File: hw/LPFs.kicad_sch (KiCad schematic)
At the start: 26 parts, among them K201 G6K-2, K202 G6K-2, K203 G6K-2, Q201 2N7002H, Q202 2N7002H, Q203 2N7002H

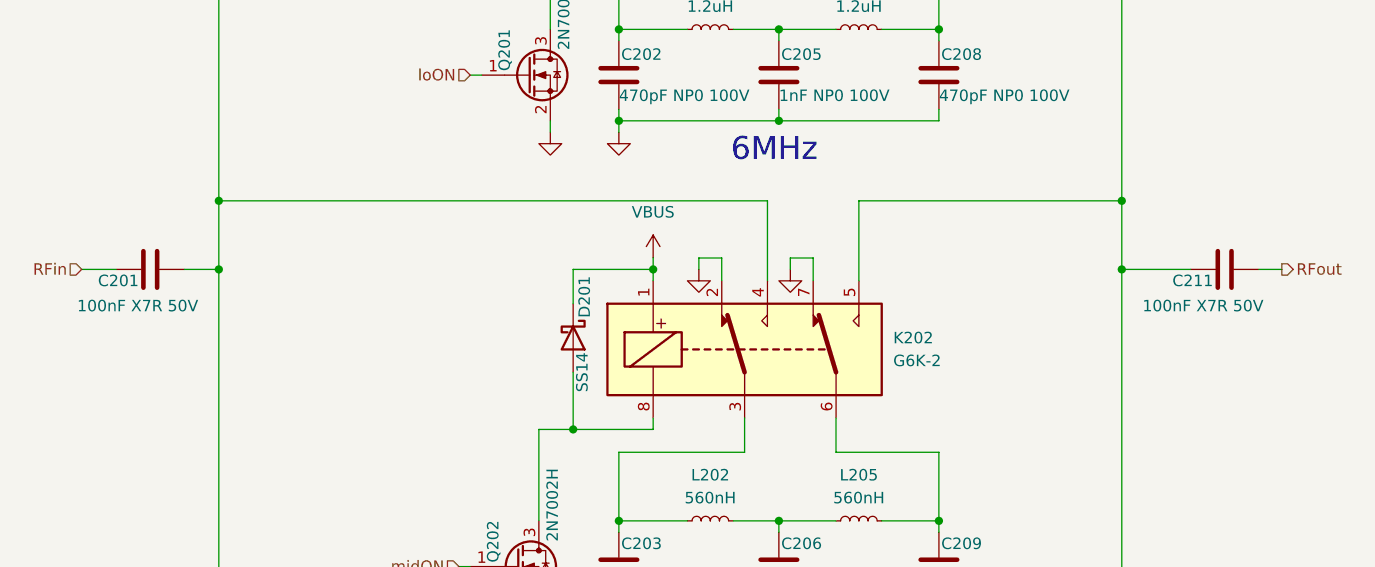
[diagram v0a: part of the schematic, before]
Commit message: Timing now closes at 121MHz. But output still does not produce any signal on my scope. Shit.
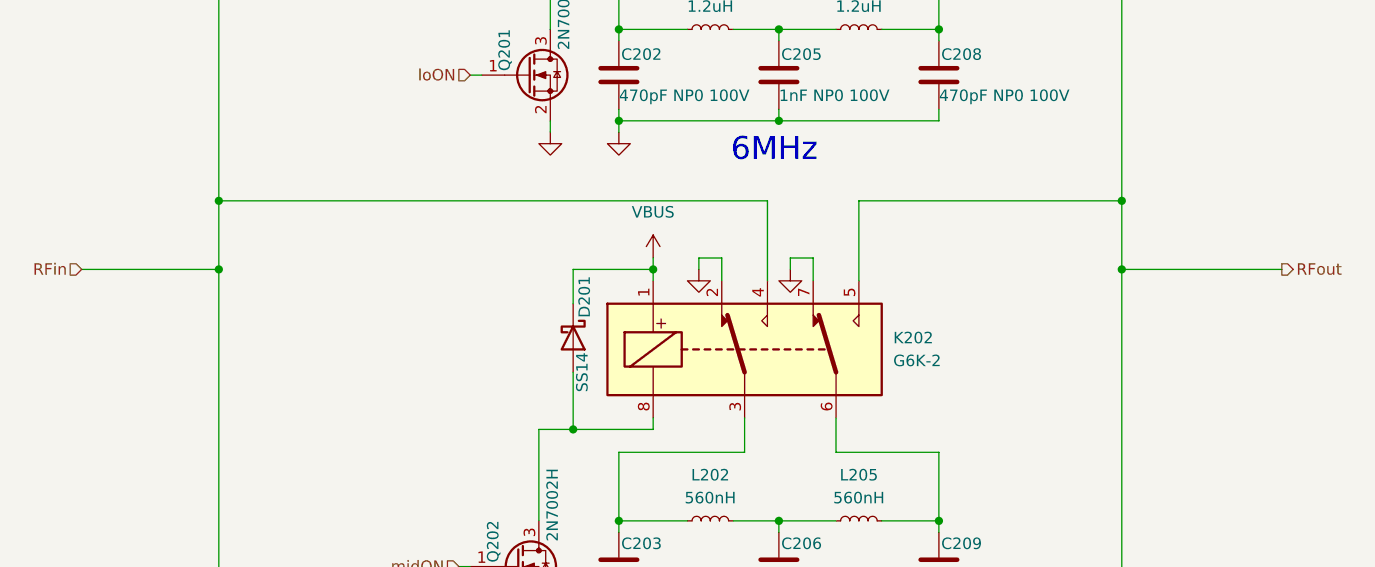
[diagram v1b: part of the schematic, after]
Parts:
- removed C201, C211: 100nF X7R 50V, Capacitor_SMD:C_0603_1608Metric, symbol Device:C
- L201, L204: MPN CW252016-1R2J -> 1008LS-122XJR; Mouser Part Number 1008LS-222 -> (none)
- L202, L205: MFG muRata -> (none); MPN LQW2UASR56G00L -> 1008CS-561X; Mouser Part Number 0805CS-391XGLC -> (none); Mouser_PN 81-LQW2UASR56G00L -> (none)
- L203, L206: MFG Bourns -> (none); MPN CW252016-R27J -> 1008CS-271XGRC; Mouser Part Number 0805CS-271 XGLC -> (none); Mouser_PN 652-CW252016-R27J -> 994-1008CS-271XGRC
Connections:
- net RFin: now also K201.4, K202.4, K203.4
- net RFout: now also K201.5, K202.5, K203.5
